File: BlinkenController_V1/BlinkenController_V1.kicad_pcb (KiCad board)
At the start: 2 copper layers, 149.5 x 64 mm, 48 parts, among them J1 Conn_01x02_Socket, J2 Conn_01x08_Socket, J4 Conn_01x03_Socket, J5 6P6C, J6 6P6C, J7 Conn_01x04_Pin, J8 Conn_01x06_Socket, SW1 SW_DIP_x01, SW2 SW_Push, SW3 SW_Push, SW4 SW_Push, SW5 SW_Push, SW6 SW_Push, U1 Pico, U2 MAX232, U3 TL331, U4 MAX3485

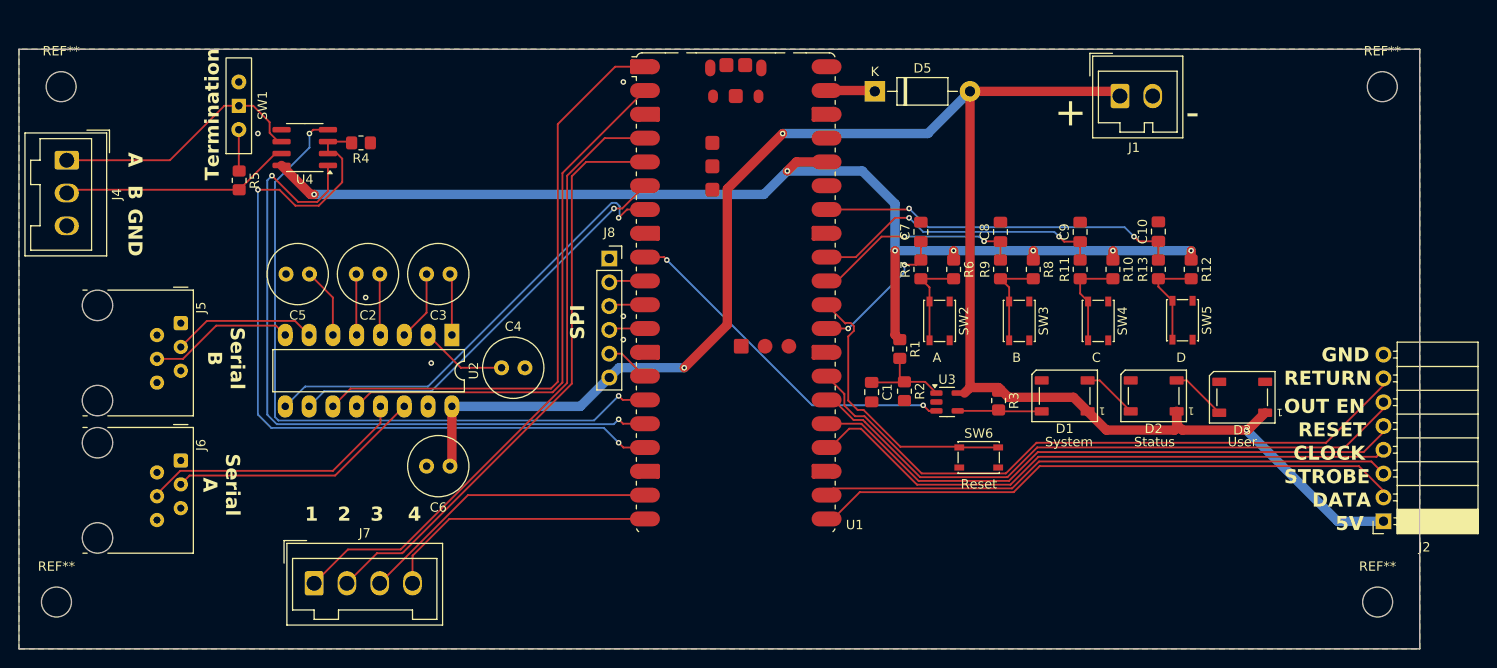
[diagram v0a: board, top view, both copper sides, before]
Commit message: Improved board density
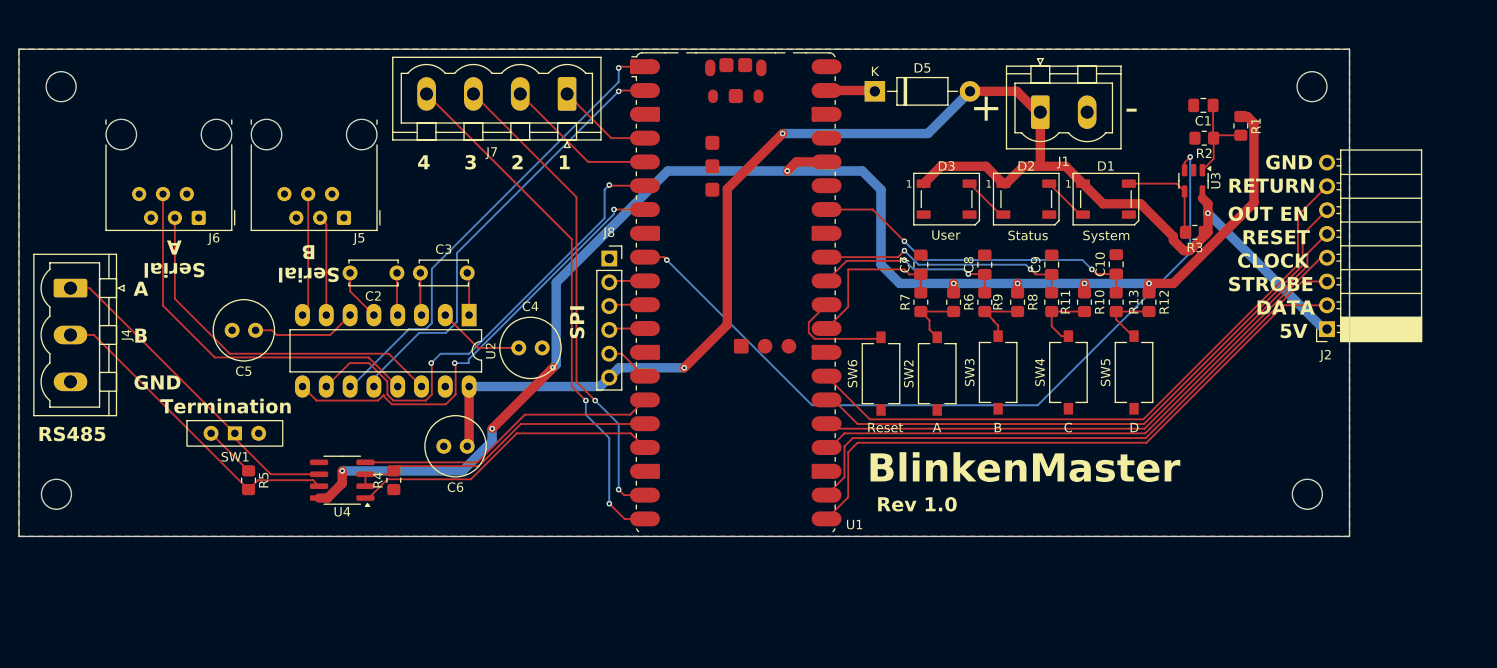
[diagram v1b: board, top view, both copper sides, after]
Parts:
- C2: footprint Capacitor_THT:C_Radial_D6.3mm_H7.0mm_P2.50mm -> Capacitor_THT:C_Disc_D5.0mm_W2.5mm_P5.00mm
- C3: footprint Capacitor_THT:C_Radial_D6.3mm_H5.0mm_P2.50mm -> Capacitor_THT:C_Disc_D5.0mm_W2.5mm_P5.00mm
- J1: footprint Connector_Wago:Wago_734-132_1x02_P3.50mm_Vertical -> Connector_Phoenix_MSTB:PhoenixContact_MSTBVA_2,5_2-G_1x02_P5.00mm_Vertical
- J4: footprint Connector_Wago:Wago_734-133_1x03_P3.50mm_Vertical -> Connector_Phoenix_MSTB:PhoenixContact_MSTBVA_2,5_3-G_1x03_P5.00mm_Vertical
- J7: footprint Connector_Wago:Wago_734-134_1x04_P3.50mm_Vertical -> Connector_Phoenix_MSTB:PhoenixContact_MSTBVA_2,5_4-G_1x04_P5.00mm_Vertical
- SW2, SW3, SW4, SW5, SW6: footprint Button_Switch_SMD:SW_SPST_PTS810 -> Button_Switch_SMD:SW_Tactile_SPST_NO_Straight_CK_PTS636Sx25SMTRLFS
- moved J7 58.8 mm to (109.0, 54.8), turned to 180 degrees
- moved C1 46.8 mm to (176.9, 56.0), turned to 180 degrees
- moved R1 43.5 mm to (180.9, 58.2)
- moved R2 41.9 mm to (177.0, 59.5), turned to 180 degrees
- moved D3 38.0 mm to (149.5, 66.0), turned to 0 degrees
- moved R4 36.2 mm to (90.5, 96.0), turned to 90 degrees
- moved U4 35.7 mm to (85.0, 96.0)
- moved U3 35.3 mm to (175.8, 64.0), turned to -90 degrees
- moved SW1 35.0 mm to (73.5, 91.0), turned to 0 degrees
- moved R5 32.0 mm to (75.0, 96.0)
- moved R3 27.6 mm to (176.0, 69.5), turned to 180 degrees
- moved J6 26.0 mm to (69.7, 68.0), turned to 180 degrees
- moved D2 25.0 mm to (158.0, 66.0), turned to 0 degrees
- moved D1 21.5 mm to (166.5, 66.0), turned to 0 degrees
- moved J2 21.4 mm to (190.1, 79.9)
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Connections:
- U1 pad 16: RS485_Rx -> RS485_Transmit
- U1 pad 17: RS485_Transmit -> RS485_Rx
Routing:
- net IN_1: track 68.0 -> 10.3 mm
- net RS485_Transmit: track 85.6 -> 33.3 mm, vias 2 -> 0
- net IN_2: track 63.4 -> 16.3 mm
- net LED_Data: track 37.9 -> 83.4 mm
- net RS485_Rx: track 77.3 -> 33.3 mm, vias 2 -> 0
- net RS485_Tx: track 74.8 -> 32.6 mm, vias 2 -> 0
- net +5V: track 190.0 -> 154.9 mm
- net +3.3V: track 124.1 -> 153.0 mm, vias 7 -> 8
- net IN_4: track 29.4 -> 56.3 mm, vias 0 -> 2
- net IN_3: track 32.2 -> 51.7 mm, vias 0 -> 2
- net Reset_CPU: track 29.7 -> 11.8 mm
- net TxD_ttl_A: track 64.4 -> 49.9 mm, vias 0 -> 1
- net TxD_A: track 27.3 -> 38.8 mm
- net RxD_A: track 29.0 -> 40.5 mm
- net RxD_ttl_A: track 57.8 -> 46.8 mm, vias 0 -> 1
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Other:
- board size 149.5 x 64 mm -> 142 x 52 mm
- board text added: "BlinkenMaster"
- board text added: "RS485"
- board text added: "Rev 1.0"
